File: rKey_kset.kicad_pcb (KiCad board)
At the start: 2 copper layers, 40.4 x 45.7 mm, 25 parts, among them J1 Conn_01x08, Q1 BC337, Q2 BC337, Q3 BC337, Q4 BC337, Q5 BC337, Q6 BC337

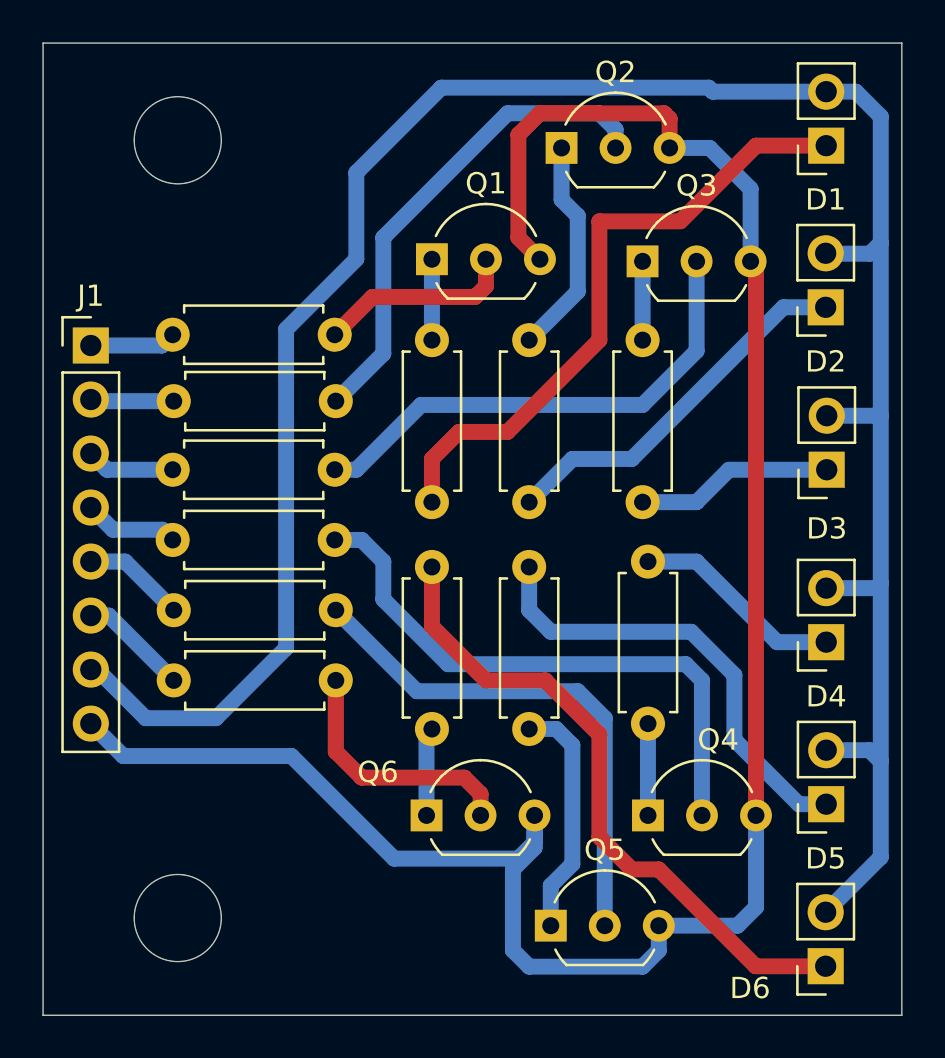
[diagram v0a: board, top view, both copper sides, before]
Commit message: Layout enhancement
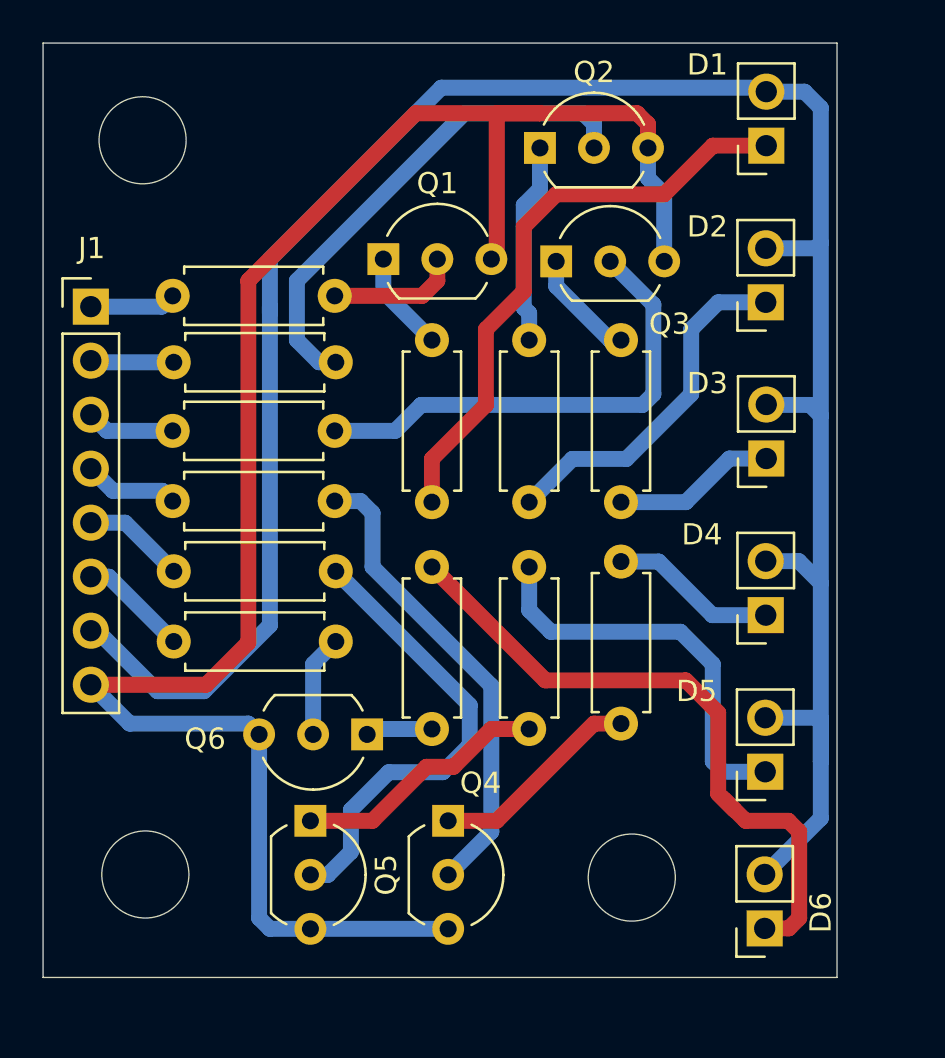
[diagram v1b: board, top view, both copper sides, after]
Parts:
- moved Q5 12.3 mm to (122.3, 102.4), turned to -90 degrees
- moved Q4 9.40 mm to (128.8, 102.4), turned to -90 degrees
- moved Q6 4.72 mm to (125.0, 98.3), turned to 180 degrees
- moved Q3 4.06 mm to (133.9, 76.1)
- moved D6 3.38 mm to (143.7, 107.4)
- moved D5 3.25 mm to (143.7, 100.1)
- moved D4 3.11 mm to (143.7, 92.7)
- moved D3 2.89 mm to (143.7, 85.3)
- moved D2 2.83 mm to (143.7, 78.0)
- moved D1 2.82 mm to (143.7, 70.6)
- moved Q1 2.29 mm to (125.7, 75.9)
- moved J1 1.83 mm to (112.0, 78.2)
- moved R2 1.83 mm to (115.9, 80.8)
- moved R4 1.83 mm to (115.8, 84.0)
- moved R7 1.83 mm to (115.8, 87.3)
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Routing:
- net GND: track 99.2 -> 89.9 mm
- net Net-(Q6-Pad2): track 12.0 -> 4.81 mm
- net Net-(Q4-Pad1): track 4.32 -> 10.0 mm
- net Net-(Q4-Pad2): track 27.4 -> 22.2 mm
- net Net-(Q1-Pad2): track 9.32 -> 6.14 mm
- net Net-(D1-Pad2): track 111.4 -> 108.3 mm
- net Net-(D5-Pad1): track 21.6 -> 19.0 mm
- net Net-(Q5-Pad2): track 24.5 -> 22.0 mm
- net Net-(D1-Pad1): track 29.9 -> 27.7 mm
- net Net-(D4-Pad1): track 9.95 -> 7.85 mm
- net Net-(D3-Pad1): track 9.29 -> 7.68 mm
- net Net-(Q3-Pad1): track 3.70 -> 5.26 mm
- net Net-(Q6-Pad1): track 4.38 -> 3.15 mm
- net Net-(Q1-Pad1): track 3.80 -> 4.76 mm
- net Net-(D2-Pad1): track 17.7 -> 16.8 mm
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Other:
- board size 40.4 x 45.7 mm -> 37.3 x 43.9 mm
